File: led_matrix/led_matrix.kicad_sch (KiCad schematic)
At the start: 12 parts, among them J101 Conn_02x08_Odd_Even, J102 Conn_01x02, U101 74HC245, U102 74HC245, U103 74154, U104 74154, U105 Inverter_Schmitt_Dual

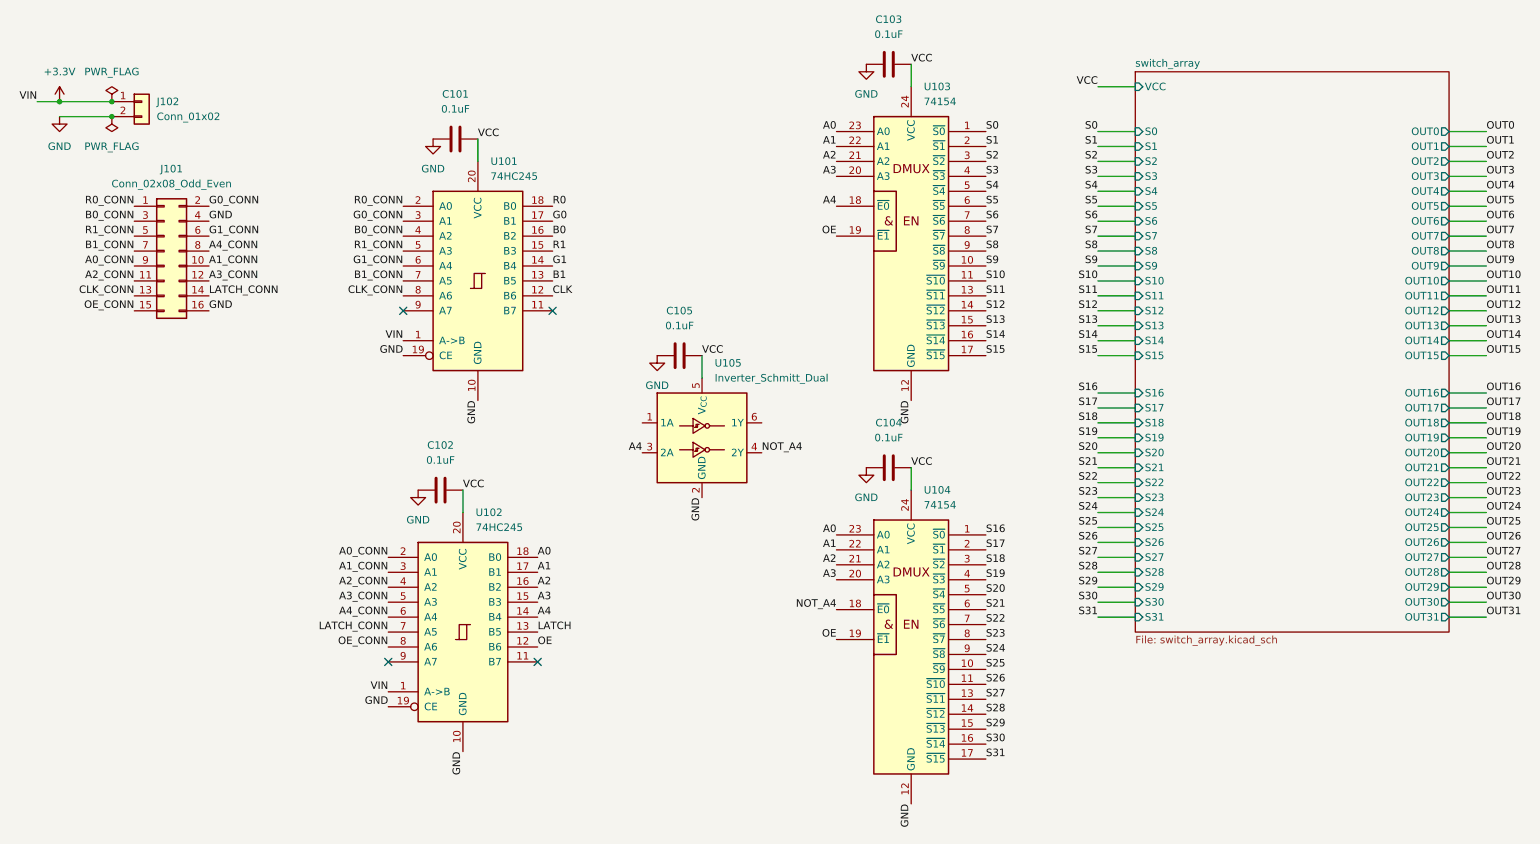
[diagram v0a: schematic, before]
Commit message: abstract input sanitation
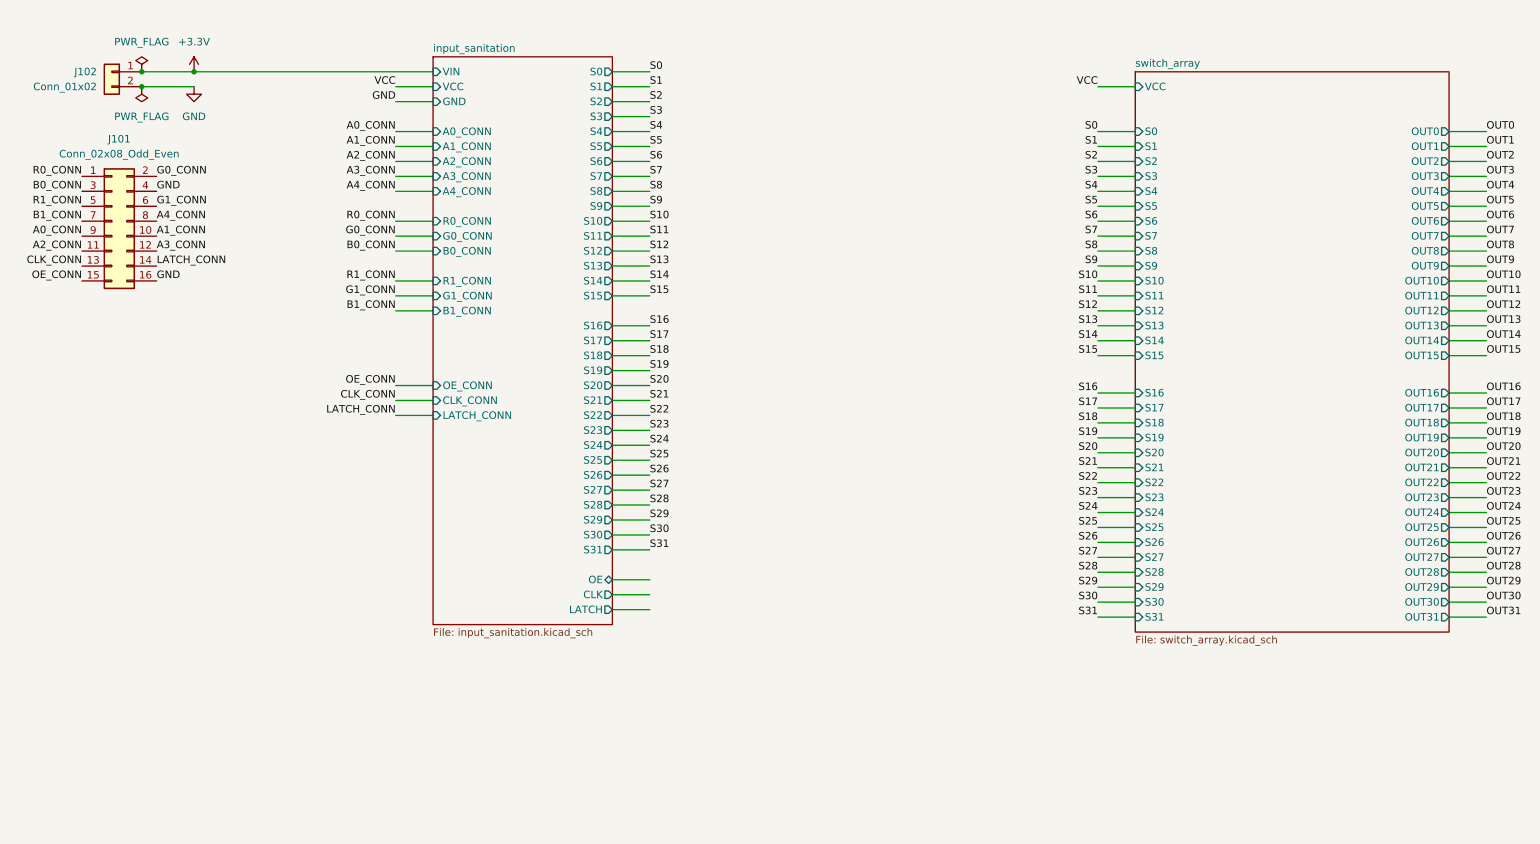
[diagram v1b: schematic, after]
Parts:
- removed C101, C102, C103, C104, C105: 0.1uF, symbol Device:C
- removed U101, U102: 74HC245, symbol 74xx:74HC245
- removed U103, U104: 74154, symbol 74xx_IEEE:74154
- removed U105: Inverter_Schmitt_Dual, symbol 74xGxx:Inverter_Schmitt_Dual
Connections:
- no-connect marks 4 -> 0
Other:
- added sheet input_sanitation (input_sanitation.kicad_sch)
- moved on the sheet: J101, J102
